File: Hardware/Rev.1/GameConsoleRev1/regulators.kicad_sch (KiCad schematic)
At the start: 13 parts, among them SW11 SW_SPDT, U4 AMS1117-3.3, U8 TLV61070ADBV

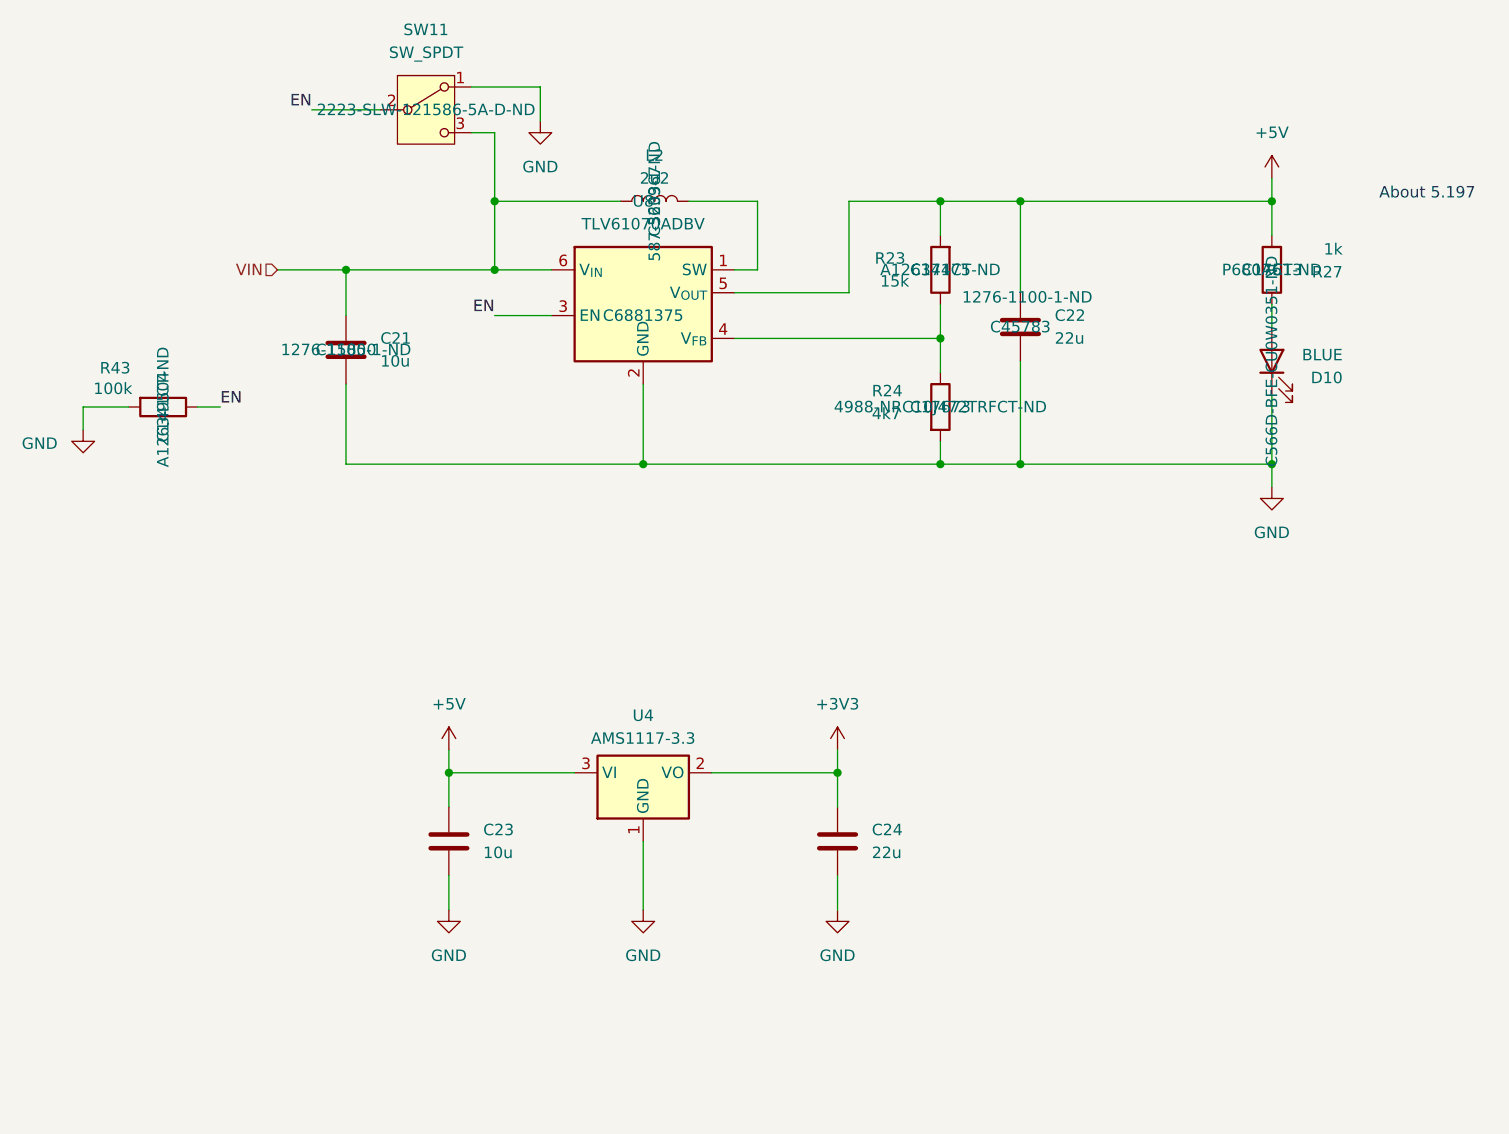
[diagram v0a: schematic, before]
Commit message: A
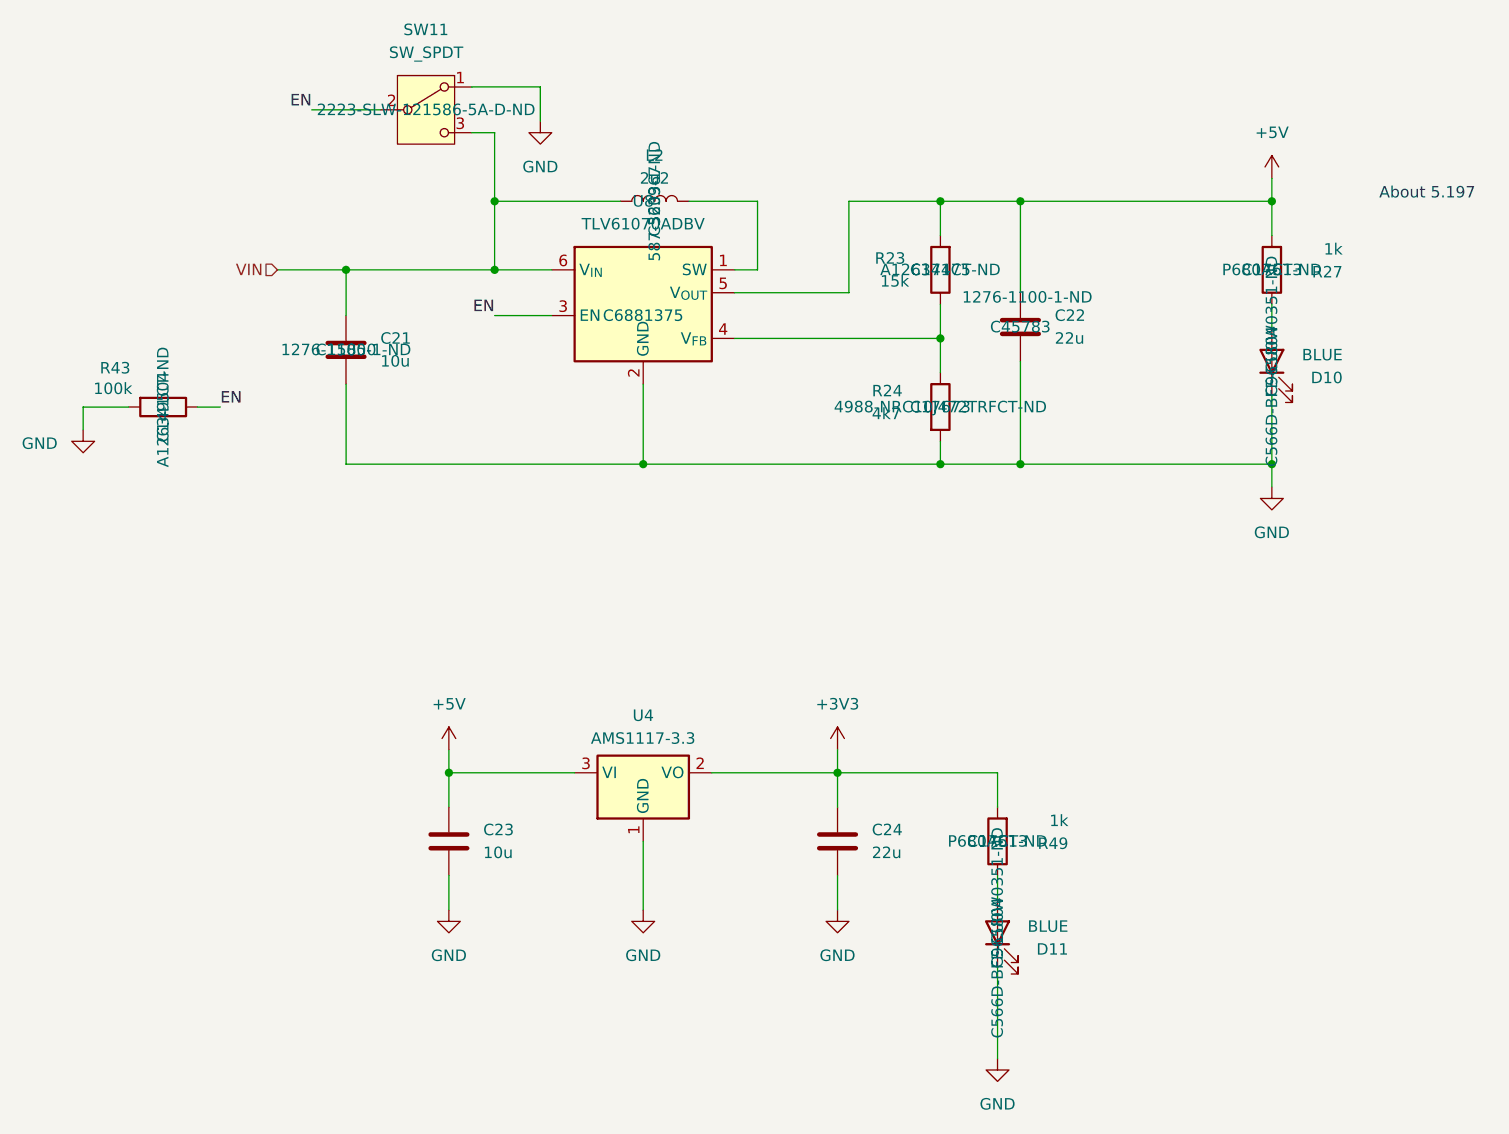
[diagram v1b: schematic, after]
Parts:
- added D11: BLUE, LED_SMD:LED_0603_1608Metric, symbol SparkFun-LED:LED
- added R49: 1k, Resistor_SMD:R_0805_2012Metric, symbol Device:R
- D10: LCSC (none) -> C965804
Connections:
- net +3V3: now also R49.2
- net GND: now also D11.1 (K)
- new net: D11.2 (A), R49.1
